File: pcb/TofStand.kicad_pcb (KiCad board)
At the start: 2 copper layers, 38.2 x 72.9 mm, 77 parts, among them SW2 SWITCH_H, U1 L6470, U2 USBLC6

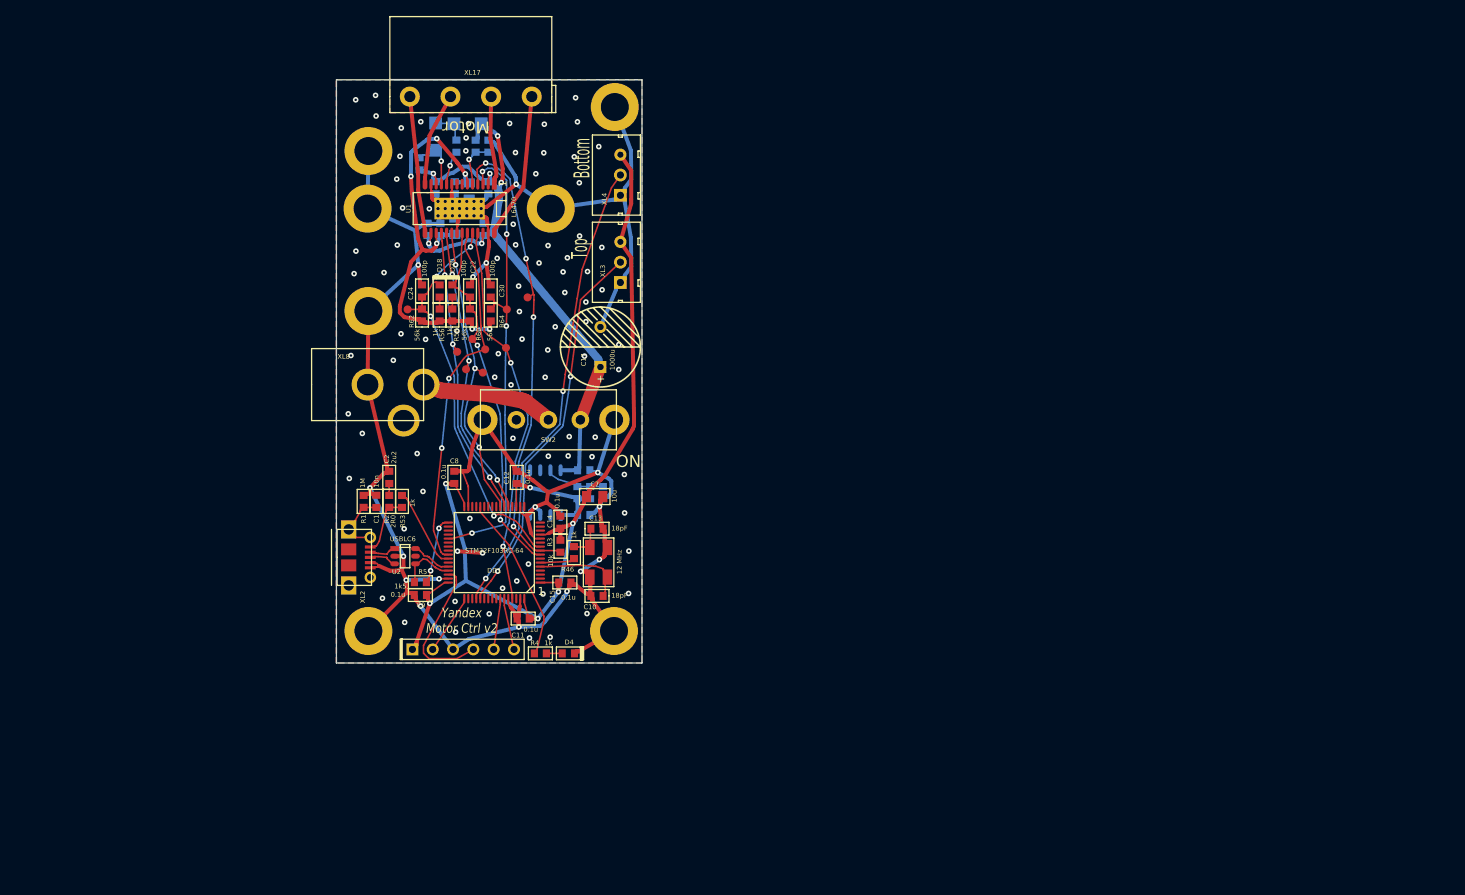
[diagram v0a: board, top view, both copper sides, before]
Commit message: PCB sent to factory
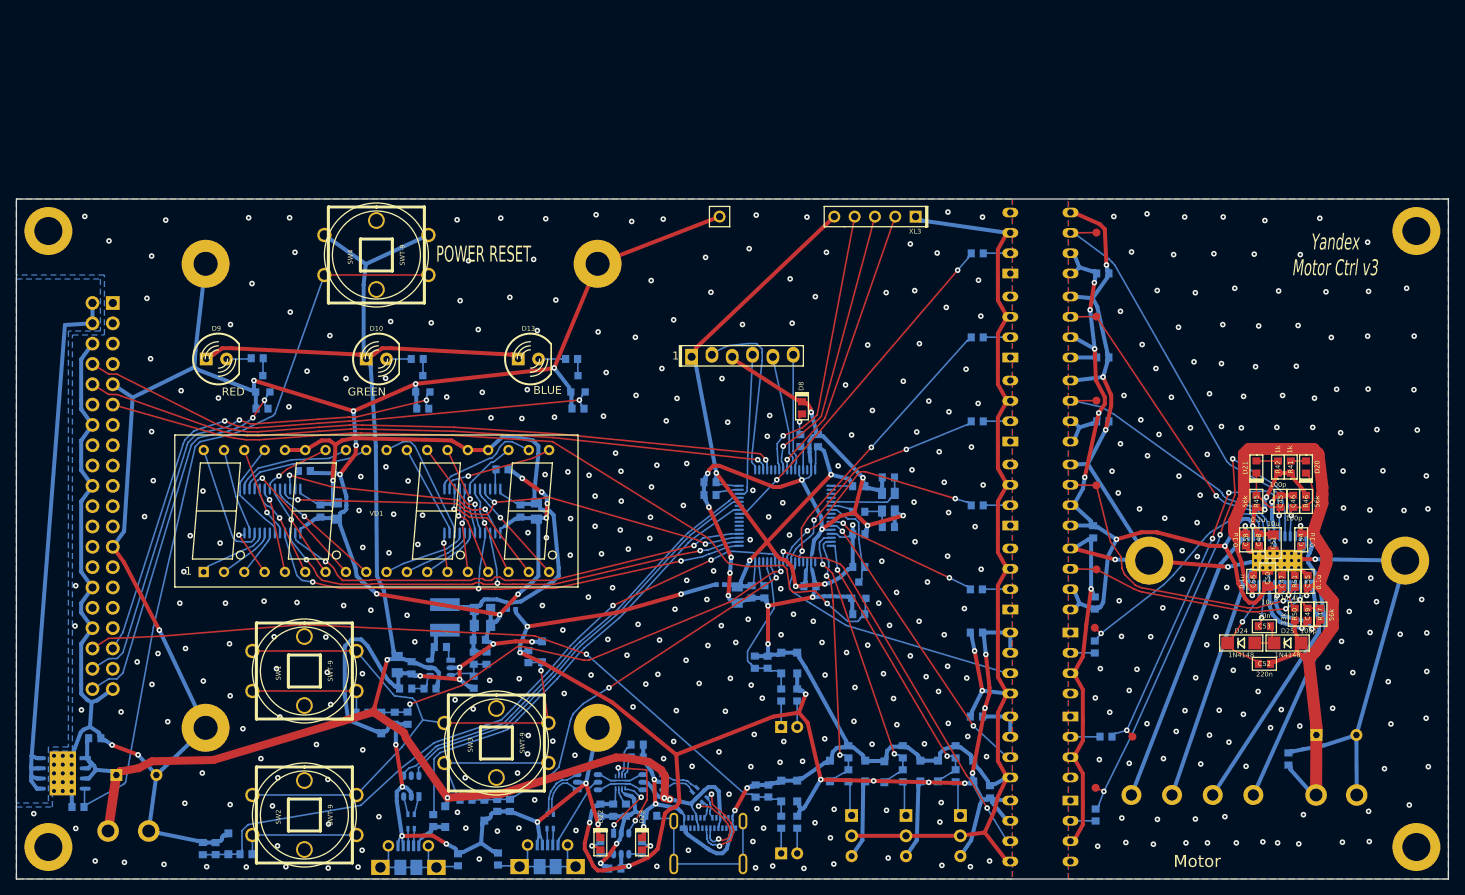
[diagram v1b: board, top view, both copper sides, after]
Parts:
- removed HOLE10, HOLE8: HOLE_METALLED, PCB:Hole3_5_out6mm
- removed R52: 12k, Resistors:RES_0603
- removed R53, R56, R58: 1k, Resistors:RES_0603
- removed R60, R62, R64: 56k, Resistors:RES_0603
- removed R68: 33k, Resistors:RES_0603
- removed R69: 4k7, Resistors:RES_0603
- removed TP4: TESTPOINT, PCB:TESTPOINT_1MM
- removed XL17: CONN_4, Connectors:TermiBlockHeader_508_x4_R
- added C20: 10u, Capacitors:CAP_0805, B.Cu at (86.3, 111.3)
- added C21: 10u, Capacitors:CAP_0805, B.Cu at (86.3, 109.3)
- added C23: 0.1u, Capacitors:CAP_0603_Silks, B.Cu at (120.4, 132.0)
- added C25: 0.1u, Capacitors:CAP_0603_Silks, B.Cu at (76.9, 122.9)
- added C28: 0.1u, Capacitors:CAP_0603_Silks, B.Cu at (163.8, 67.3)
- added C29: 0.1u, Capacitors:CAP_0603_Silks, B.Cu at (163.8, 77.8)
- added C3: 0.1u, Capacitors:CAP_0603_Silks, B.Cu at (37.8, 125.4)
- added C31: 0.1u, Capacitors:CAP_0603_Silks, B.Cu at (149.7, 132.1)
- added C34: 0.1u, Capacitors:CAP_0603_Silks, B.Cu at (162.6, 99.6)
- added C35: 0.1u, Capacitors:CAP_0603_Silks, B.Cu at (162.8, 108.5)
- added C38: 0.1u, Capacitors:CAP_0603_Silks, B.Cu at (105.6, 126.2)
- added C39: 10u, Capacitors:CAP_0805, B.Cu at (68.0, 97.0)
- added C4: 18pF, Capacitors:CAP_0603_Silks, B.Cu at (137.0, 99.0)
- added C41: 1u, Capacitors:CAP_0603_Silks, B.Cu at (102.8, 141.7)
- added C43: 0.1u, Capacitors:CAP_0603_Silks, B.Cu at (104.2, 134.4)
- added C45: 100p, Capacitors:CAP_0603_Silks, F.Cu at (186.0, 95.8)
- added C47: 0.1u, Capacitors:CAP_0603_Silks, F.Cu at (186.2, 105.8)
- added C48: 0.1u, Capacitors:CAP_0603_Silks, F.Cu at (183.3, 100.6)
- added C49: 100p, Capacitors:CAP_0603_Silks, F.Cu at (189.4, 109.9)
- added C5: 0.1u, Capacitors:CAP_0603_Silks, B.Cu at (119.9, 107.1)
- added C50: 10u, Capacitors:CAP_0805, F.Cu at (184.4, 105.4)
- added C51: 10u, Capacitors:CAP_0805, F.Cu at (185.1, 101.0)
- added C52: 220n, Capacitors:CAP_0603_Silks, F.Cu at (184.0, 116.1)
- added C53: 10n, Capacitors:CAP_0603_Silks, F.Cu at (184.0, 111.4)
- added C54: 0.1u, Capacitors:CAP_0603_Silks, F.Cu at (188.6, 100.6)
- added C55: 0.1u, Capacitors:CAP_0603_Silks, F.Cu at (189.4, 105.8)
- added C56: 0.1u, Capacitors:CAP_0603_Silks, F.Cu at (182.6, 105.8)
- added C57: 1000u, Capacitors:CAP_10xxR, B.Cu at (193.0, 125.0)
- added C58: 0.1u, Capacitors:CAP_0603_Silks, F.Cu at (181.7, 100.6)
- added C59: 0.1u, Capacitors:CAP_0603_Silks, B.Cu at (187.0, 128.0)
- added C6: 1000u, Capacitors:CAP_10xxR, B.Cu at (43.0, 130.0)
- added D1: PESD3V3, Diodes:SOD323, B.Cu at (134.1, 129.5)
- added D10: LED, LEDs:LED_Through-Hole-5mm, F.Cu at (73.0, 78.0)
- added D11: PESD3V3, Diodes:SOD323, B.Cu at (123.6, 132.0)
- added D12: PESD3V3, Diodes:SOD323, B.Cu at (125.6, 132.0)
- added D13: LED, LEDs:LED_Through-Hole-5mm, F.Cu at (92.0, 78.0)
- added D14: PESD3V3, Diodes:SOD323, B.Cu at (93.7, 114.6)
- added D15: PESD3V3, Diodes:SOD323, B.Cu at (73.6, 123.5)
- added D16: PESD3V3, Diodes:SOD323, B.Cu at (54.5, 138.6)
- added D17: PESD3V3, Diodes:SOD323, B.Cu at (86.5, 134.4)
- added D19: PESD3V3, Diodes:SOD323, B.Cu at (125.6, 116.0)
- added D2: PESD3V3, Diodes:SOD323, B.Cu at (141.0, 129.5)
- added D21: LED, LEDs:LED_0603, F.Cu at (183.0, 91.5)
- added D22: LED, LEDs:LED_0603, F.Cu at (101.0, 138.6)
- added D24: 1N4148, Diodes:SOD80C, F.Cu at (181.1, 113.5)
- added D3: PESD3V3, Diodes:SOD323, B.Cu at (147.6, 129.5)
- added D5: PESD3V3, Diodes:SOD323, B.Cu at (129.7, 129.5)
- added D6: PESD3V3, Diodes:SOD323, B.Cu at (136.5, 129.6)
- added D7: PESD3V3, Diodes:SOD323, B.Cu at (143.2, 129.5)
- added D8: LED, LEDs:LED_0603, F.Cu at (126.2, 84.1)
- added D9: LED, LEDs:LED_Through-Hole-5mm, F.Cu at (53.0, 78.0)
- added DA2: Optocoupler_6N137, DIP:DIP-8_296_ELL, B.Cu at (156.0, 116.0)
- added DA3: Optocoupler_6N137, DIP:DIP-8_296_ELL, B.Cu at (156.0, 63.5)
- added DA4: Optocoupler_6N137, DIP:DIP-8_296_ELL, B.Cu at (156.0, 74.0)
- added DA5: Optocoupler_6N137, DIP:DIP-8_296_ELL, B.Cu at (156.0, 84.5)
- added DA6: Optocoupler_6N137, DIP:DIP-8_296_ELL, B.Cu at (156.0, 137.0)
- added DA7: Optocoupler_6N137, DIP:DIP-8_296_ELL, B.Cu at (156.0, 126.5)
- added DA8: Optocoupler_6N137, DIP:DIP-8_296_ELL, B.Cu at (156.0, 95.0)
- added DA9: Optocoupler_6N137, DIP:DIP-8_296_ELL, B.Cu at (156.0, 105.5)
- added DD2: ICN2595, SO_DIL_TSSOP:TSSOP24_150_0635, B.Cu at (60.0, 97.0)
- added DD3: ICN2595, SO_DIL_TSSOP:TSSOP24_150_0635, B.Cu at (85.0, 97.0)
- added DD4: 74LVC2G17, SOT:SOT23-6, B.Cu at (103.6, 138.6)
- added DD5: TUSB211, QFN_DFN:X2QFN_12, B.Cu at (103.5, 130.9)
- added HOLE3: HOLE_METALLED, PCB:Hole3_5_out6mm, F.Cu at (203.0, 62.0)
- added L1: BLM21PG221SN1D, Inductors:IND_0603, B.Cu at (83.2, 140.6)
- added L2: BLM15AG102, Inductors:IND_0402, B.Cu at (116.0, 106.2)
- added L3: 90R, Inductors:DLW21SN, B.Cu at (77.3, 135.8)
- added L4: 2R2, Inductors:IND_1515, B.Cu at (81.6, 110.3)
- added L5: Choke, Inductors:IND_0402, B.Cu at (89.9, 109.3)
- added L6: BLM21PG221SN1D, Inductors:IND_0603, B.Cu at (107.3, 135.1)
- added L7: 90R, Inductors:DLW21SN, B.Cu at (113.4, 132.5)
- added L8: 90R, Inductors:DLW21SN, B.Cu at (94.7, 135.8)
- added L9: BLM21PG221SN1D, Inductors:IND_0603, B.Cu at (88.2, 140.5)
- added Q1: 2N7002, SOT:SOT23-3, B.Cu at (58.8, 81.1)
- added Q2: 2N7002, SOT:SOT23-3, B.Cu at (78.8, 81.1)
- added Q3: 2N7002, SOT:SOT23-3, B.Cu at (98.2, 81.1)
- added Q4: IRF9321, SO_DIL_TSSOP:SO8HEATSINK, B.Cu at (33.8, 129.8)
- added Q5: 2N7002, SOT:SOT23-3, B.Cu at (133.3, 106.9)
- added R10: 22k, Resistors:RES_0603, B.Cu at (85.2, 118.4)
- added R11: 100k, Resistors:RES_0603, B.Cu at (78.8, 84.2)
- added R12: 1k, Resistors:RES_0603, B.Cu at (125.6, 135.9)
- added R13: 1k, Resistors:RES_0603, B.Cu at (123.6, 135.9)
- added R14: 1k, Resistors:RES_0603, B.Cu at (78.1, 78.0)
- added R15: 1k, Resistors:RES_0603, B.Cu at (80.1, 135.7)
- added R16: 100k, Resistors:RES_0603, B.Cu at (98.2, 84.2)
- added R17: 100k, Resistors:RES_0603, B.Cu at (122.0, 132.0)
- added R18: 1k, Resistors:RES_0603, B.Cu at (97.4, 78.0)
- added R19: 1k, Resistors:RES_0603, B.Cu at (92.0, 115.2)
- added R20: 1k, Resistors:RES_0603, B.Cu at (148.1, 64.8)
- added R21: 1k, Resistors:RES_0603, B.Cu at (148.1, 75.3)
- added R22: 1k, Resistors:RES_0603, B.Cu at (148.1, 85.8)
- added R23: 1k, Resistors:RES_0603, B.Cu at (71.2, 122.2)
- added R24: 1k, Resistors:RES_0603, B.Cu at (56.7, 139.9)
- added R25: 1k, Resistors:RES_0603, B.Cu at (84.2, 133.1)
- added R26: 10k, Resistors:RES_0603, B.Cu at (35.7, 134.0)
- added R27: 100k, Resistors:RES_0603, B.Cu at (75.3, 122.9)
- added R28: 100k, Resistors:RES_0603, B.Cu at (52.9, 139.2)
- added R29: 100k, Resistors:RES_0603, B.Cu at (88.1, 133.8)
- added R30: 1k, Resistors:RES_0603, B.Cu at (162.8, 114.0)
- added R31: 1k, Resistors:RES_0603, B.Cu at (125.6, 120.0)
- added R32: 1k, Resistors:RES_0603, B.Cu at (123.6, 120.0)
- added R33: 1k, Resistors:RES_0603, B.Cu at (148.1, 96.3)
- added R34: 1k, Resistors:RES_0603, B.Cu at (148.0, 106.8)
- added R35: 100k, Resistors:RES_0603, B.Cu at (121.9, 115.9)
- added R36: 1k, Resistors:RES_0603, B.Cu at (162.9, 135.0)
- added R37: 1k, Resistors:RES_0603, B.Cu at (164.2, 125.2)
- added R38: 1k, Resistors:RES_0603, B.Cu at (64.0, 92.0)
- added R39: 1k, Resistors:RES_0603, B.Cu at (88.7, 91.8)
- added R40: 3k9, Resistors:RES_0603, B.Cu at (105.6, 127.8)
- added R41: 1k, Resistors:RES_0603, F.Cu at (187.3, 91.5)
- added R42: 1k, Resistors:RES_0603, F.Cu at (185.7, 91.5)
- added R43: 1k, Resistors:RES_0603, B.Cu at (101.0, 139.1)
- added R44: 1k, Resistors:RES_0603, B.Cu at (106.2, 139.1)
- added R45: 56k, Resistors:RES_0603, F.Cu at (183.0, 95.8)
- added R47: 56k, Resistors:RES_0603, F.Cu at (191.0, 109.9)
- added R48: 100k, Resistors:RES_0603, B.Cu at (133.3, 109.9)
- added R49: 10k, Resistors:RES_0603, B.Cu at (133.3, 104.0)
- added R50: 33k, Resistors:RES_0603, F.Cu at (187.8, 109.9)
- added R6: 1k, Resistors:RES_0603, B.Cu at (126.0, 88.2)
- added R7: 100k, Resistors:RES_0603, B.Cu at (58.7, 84.2)
- added R8: 1k, Resistors:RES_0603, B.Cu at (58.1, 77.9)
- added R9: 100k, Resistors:RES_0603, B.Cu at (85.2, 115.4)
- added SW1: SWT-9, BtnsSwitches:BTN_SWT9, F.Cu at (64.0, 117.0)
- added SW3: SWT-9, BtnsSwitches:BTN_SWT9, F.Cu at (88.0, 126.0)
- added SW4: SWT-9, BtnsSwitches:BTN_SWT9, F.Cu at (73.0, 65.0)
- added U3: USBLC6, SOT:SOT23-6, B.Cu at (99.4, 130.9)
- added U4: L6470, SO_DIL_TSSOP:HTSSOP28, B.Cu at (185.6, 103.2)
- added VCap1: 2.2u, Capacitors:CAP_0603_Silks, B.Cu at (121.5, 107.1)
- added VCap2: 2.2u, Capacitors:CAP_0603_Silks, B.Cu at (114.7, 95.0)
- added VD1: 7SEGx4_CA, Display:7Segx4, F.Cu at (73.0, 97.0)
- added XL10: CONN_2, Connectors:WB-02(MW-2M), B.Cu at (124.6, 124.0)
- added XL11: RASPBERRY_3B, Installation:RaspberryPi3, B.Cu at (40.0, 71.0)
- added XL12: CONN_4, Connectors:TermiBlockHeader_508_x4_R, B.Cu at (175.0, 132.5)
- added XL13: USB_MICRO, Connectors:USBmicro_MOLEX_1050170001, B.Cu at (94.4, 142.9)
- added XL14: CONN_2, Connectors:2ZHDRC-02P, B.Cu at (193.0, 132.5)
- added XL15: CONN_1, Connectors:PLS-1Rnd, B.Cu at (115.9, 60.2)
- added XL5: CONN_3, Connectors:W03_Pitch_2d54, B.Cu at (139.2, 137.6)
- added XL6: CONN_3, Connectors:W03_Pitch_2d54, B.Cu at (146.0, 137.6)
- added XL7: USB_MICRO, Connectors:USBmicro_MOLEX_1050170001, B.Cu at (77.0, 143.0)
- added XL9: USB_C, Connectors:USB_C_MOLEX_1054500101, B.Cu at (114.5, 142.9)
- C1: value 10n -> 18pF; footprint Capacitors:CAP_0603 -> Capacitors:CAP_0603_Silks; moved to B.Cu
- C10: value 18pF -> 10nF; footprint Capacitors:CAP_0603 -> Capacitors:CAP_0603_Silks; moved to B.Cu
- C11, C9: value 0.1u -> 10nF; footprint Capacitors:CAP_0603 -> Capacitors:CAP_0603_Silks; moved to B.Cu
- C12, C8: footprint Capacitors:CAP_0603 -> Capacitors:CAP_0603_Silks; moved to B.Cu
- C13: value 18pF -> 10u; footprint Capacitors:CAP_0603 -> Capacitors:CAP_0805; moved to B.Cu
- C14, C15: value 0.1u -> 1u; footprint Capacitors:CAP_0603 -> Capacitors:CAP_0603_Silks; moved to B.Cu
- C16, C26, C27: footprint Capacitors:CAP_0603 -> Capacitors:CAP_0603_Silks
- C17: value 1000u -> 0.1u; footprint Capacitors:CAP_10xxR -> Capacitors:CAP_0603_Silks; moved to B.Cu
- C18: value 1000pF -> 0.1u; footprint Capacitors:CAP_0603 -> Capacitors:CAP_0603_Silks
- C19: value 1u -> 27pF; footprint Capacitors:CAP_0603 -> Capacitors:CAP_0603_Silks
- C2: value 2u2 -> 10u; footprint Capacitors:CAP_0603 -> Capacitors:CAP_0805; moved to B.Cu
- C22, C24, C30: value 100p -> 0.1u; footprint Capacitors:CAP_0603 -> Capacitors:CAP_0603_Silks; moved to B.Cu
- C32, C33: value 10u -> 0.1u; footprint Capacitors:CAP_0805 -> Capacitors:CAP_0603_Silks
- C36: value 220n -> 0.1u; footprint Capacitors:CAP_0603 -> Capacitors:CAP_0603_Silks
- C37: value 10n -> 0.1u; footprint Capacitors:CAP_0603 -> Capacitors:CAP_0603_Silks
- C40: value 0.1u -> 10u; footprint Capacitors:CAP_0603 -> Capacitors:CAP_0805
- C42: value 0.1u -> 10n; footprint Capacitors:CAP_0603 -> Capacitors:CAP_0603_Silks
- C44: value 0.1u -> 1u; footprint Capacitors:CAP_0603 -> Capacitors:CAP_0603_Silks
- C46: value 0.1u -> 100p; footprint Capacitors:CAP_0603 -> Capacitors:CAP_0603_Silks; moved to F.Cu
- C7: value 10u -> 0.1u; footprint Capacitors:CAP_0805 -> Capacitors:CAP_0603_Silks; moved to B.Cu
- D18: value LED -> PESD3V3; footprint LEDs:LED_0603 -> Diodes:SOD323; moved to B.Cu
- D23: value 1N4148 -> LED; footprint Diodes:SOD80C -> LEDs:LED_0603; moved to F.Cu
- D25: moved to F.Cu
- D4: value LED -> PMEG2020; footprint LEDs:LED_0603 -> Diodes:SOD323; moved to B.Cu
- DA1: value LP2951 -> SY8120; footprint SO_DIL_TSSOP:SO8_150MIL -> SOT:SOT23-6
- DD1: value STM32F103RC-64 -> STM32F205Rx-64; moved to B.Cu
- R1: value 1M -> 1k; moved to B.Cu
- R2: value 2R0 -> 1k; moved to B.Cu
- R3: value 10k -> 1k; moved to B.Cu
- R4, U2, XL4: moved to B.Cu
- R46: value 1k -> 56k
- R5: value 1k5 -> 56k; moved to B.Cu
- R51: value 20k -> 4k7; moved to F.Cu
- SW2: value SWITCH_H -> SWT-9; footprint BtnsSwitches:SW_SS9 -> BtnsSwitches:BTN_SWT9
- U1: value L6470 -> USBLC6; footprint SO_DIL_TSSOP:HTSSOP28 -> SOT:SOT23-6; moved to B.Cu
- XL1: value CONN_6 -> CONN_2; footprint Connectors:PLS-6 -> Connectors:2ZHDRC-02P; moved to B.Cu
- XL2: value USB_MICRO -> CONN_6; footprint Connectors:USBmicro_MOLEX_1050170001 -> Connectors:PLS-6_LOCK
- XL3: value CONN_3 -> CONN_5; footprint Connectors:W03_Pitch_2d54 -> Connectors:PLS-5
- XL8: value BARREL_SOCKET -> CONN_2; footprint Connectors:Barrel -> Connectors:WB-02(MW-2M); moved to B.Cu
- XTAL1: footprint Quartz:0503x4-4 -> Quartz:03225C4; moved to B.Cu
- moved HOLE6 134.4 mm to (203.0, 139.0), turned to 0 degrees
- moved HOLE2 129.9 mm to (201.6, 103.2)
- moved D25 121.3 mm to (186.9, 113.5)
- moved C46 113.4 mm to (187.6, 95.8)
- moved D20 108.9 mm to (189.2, 91.5), turned to -90 degrees
- moved TP3 104.7 mm to (162.9, 131.6), turned to 0 degrees
- moved HOLE1 102.5 mm to (169.6, 103.2)
- moved TP1 96.3 mm to (167.5, 125.2), turned to 0 degrees
- moved HOLE4 95.8 mm to (32.0, 139.0)
- moved D23 92.1 mm to (106.2, 138.6)
- moved R46 91.7 mm to (189.2, 95.8), turned to -90 degrees
- moved C32 91.3 mm to (148.0, 122.7), turned to 180 degrees
- moved R51 90.4 mm to (187.8, 105.8)
- moved C26 88.4 mm to (51.3, 139.2), turned to 90 degrees
- moved XL4 87.5 mm to (132.4, 137.6), turned to -90 degrees
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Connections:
- C1 pad 1: GND -> Net-(C1-Pad1)
- C1 pad 2: Net-(C1-Pad2) -> GND
- C10 pad 1: Net-(C10-Pad1) -> /ENDSTOP_BOT
- C11 pad 1: +3v3 -> /ENDSTOP_TOUCH
- C12 pad 1: +3v3 -> PwrMCU
- C13 pad 1: Net-(C13-Pad1) -> +5v
- C14 pad 1: +3v3 -> +5v
- C15 pad 1: +3v3 -> PwrMCU
- C16 pad 1: +12v -> PwrMCU
- C17 pad 1: +12v -> Net-(C13-Pad1)
- C18 pad 1: +3v3 -> Net-(C19-Pad1)
- C18 pad 2: Net-(C18-Pad2) -> Net-(C19-Pad2)
- C19 pad 1: +3v3 -> /PWR_LEDS
- C19 pad 2: GND -> Net-(C23-Pad2)
- C2 pad 1: Net-(C2-Pad1) -> PwrMCU
- C22 pad 1: /BUSY/SYNC_1 -> /PWR_LEDS
- C24 pad 1: /FLAG_1 -> +3v3
- C26 pad 1: /Vdd1 -> /BtnDown
- C27 pad 1: /Vdd1 -> /BtnFast
- C30 pad 1: /STBY/RST -> VCC
- C30 pad 2: GND -> GNDPWR
- C32 pad 1: /Vdd1 -> +3v3
- C33 pad 1: /Vdd1 -> /ChClosed
- C36 pad 1: Net-(C36-Pad1) -> GND
- C36 pad 2: +12v -> /PWR_LEDS
- C37 pad 1: Net-(C37-Pad1) -> GND
- C37 pad 2: Net-(C37-Pad2) -> /PWR_LEDS
- C40 pad 1: +12v -> GND
- C40 pad 2: GND -> /PWR_LEDS
- C42 pad 1: +12v -> GND
- C42 pad 2: GND -> +3v3
- C44 pad 1: +12v -> GND
- C44 pad 2: GND -> +3v3
- C46 pad 1: +12v -> /FLAG
- C46 pad 2: GND -> GNDPWR
- C7 pad 1: +3v3 -> PwrMCU
- C8 pad 1: +3v3 -> PwrMCU
- C9 pad 1: +3v3 -> /ENDSTOP_TOP
- D18 pad A: Net-(D18-PadA) (its old number) -> GND
- D18 pad C: /FLAG_1 -> /ChClosed
- D20 pad C: /BUSY/SYNC_1 -> /FLAG
- D23 pad A: Net-(C37-Pad1) -> Net-(D21-PadA)
- D23 pad C: Net-(C36-Pad1) -> GND
- D4 pad A: Net-(D4-PadA) -> /5V_USB
- D4 pad C: GND -> +5v
- DA1 pad 1: +3v3 -> Net-(C19-Pad1)
- DA1 pad 2: (no net) -> GND
- DA1 pad 3: GND -> Net-(C23-Pad2)
- DA1 pad 4: GND -> Net-(C13-Pad1)
- DA1 pad 5: (no net) -> +5v
- DA1 pad 6: (no net) -> Net-(C19-Pad2)
- DD1 pad 1: +3v3 -> PwrMCU
- DD1 pad 10: /FLAG_1 -> /STBY/RST_MCU
- DD1 pad 11: (no net) -> /BUSY/SYNC_MCU
- DD1 pad 13: +3v3 -> PwrMCU
- DD1 pad 14: (no net) -> /ENDSTOP_BOT
- DD1 pad 15: (no net) -> /ENDSTOP_TOP
- DD1 pad 16: (no net) -> /ENDSTOP_TOUCH
- DD1 pad 19: +3v3 -> PwrMCU
- DD1 pad 21: /MOTOR_SCK -> /MOTOR_SCK_MCU
- DD1 pad 22: /MOTOR_MISO -> /MOTOR_MISO_MCU
- DD1 pad 23: /MOTOR_MOSI -> /MOTOR_MOSI_MCU
- DD1 pad 24: (no net) -> /SW_MCU
- DD1 pad 25: (no net) -> /FLAG_MCU
- DD1 pad 26: (no net) -> /BtnUp
- DD1 pad 27: (no net) -> /BtnDown
- DD1 pad 28: Net-(DD1-Pad28) -> /BtnFast
- DD1 pad 29: (no net) -> /ChClosed
- DD1 pad 31: GND -> Net-(DD1-Pad31)
- DD1 pad 32: +3v3 -> PwrMCU
- DD1 pad 33: /USB_PULLUP -> /LATCH
- DD1 pad 34: (no net) -> /CLK
- DD1 pad 35: (no net) -> /OUT_EN
- DD1 pad 36: (no net) -> /DATA_IN1
- DD1 pad 37: /STBY/RST -> (no net)
- DD1 pad 41: /MOTOR_CS -> /MOTOR_CS_MCU
- DD1 pad 47: GND -> Net-(DD1-Pad47)
- DD1 pad 48: +3v3 -> PwrMCU
- DD1 pad 5: Net-(C10-Pad1) -> Net-(C1-Pad1)
- DD1 pad 51: (no net) -> /MCU_TX_RPI_RX
- DD1 pad 52: /ENDSTOP_BOT -> /MCU_RX_RPI_TX
- DD1 pad 53: /ENDSTOP_TOP -> (no net)
- DD1 pad 55: (no net) -> /PB5
- DD1 pad 56: (no net) -> /PB4
- DD1 pad 57: (no net) -> /PB3
- DD1 pad 61: /STEP_CLK_1 -> Net-(DD1-Pad61)
- DD1 pad 64: +3v3 -> PwrMCU
- DD1 pad 7: (no net) -> /MCU_RESET
- DD1 pad 8: /BUSY/SYNC_1 -> (no net)
- DD1 pad 9: /SW_1 -> (no net)
- HOLE1 pad H: GND -> GNDPWR
- HOLE2 pad H: GND -> GNDPWR
- HOLE4 pad H: GND -> (no net)
- HOLE5 pad H: GND -> (no net)
- HOLE6 pad H: GND -> (no net)
- R1 pad 1: Net-(C1-Pad2) -> /ENDSTOP_TOP
- R1 pad 2: GND -> Net-(R1-Pad2)
- R2 pad 1: /5V_USB -> /ENDSTOP_BOT
- R2 pad 2: Net-(C2-Pad1) -> Net-(R2-Pad2)
- R3 pad 1: +3v3 -> /ENDSTOP_TOUCH
- R3 pad 2: /SW_1 -> Net-(R3-Pad2)
- R4 pad 1: Net-(DD1-Pad28) -> Net-(DD1-Pad6)
- R4 pad 2: Net-(D4-PadA) -> Net-(C4-Pad1)
- R46 pad 1: Net-(DD1-Pad6) -> VCC
- R46 pad 2: Net-(C13-Pad1) -> /FLAG
- R5 pad 1: /USB_D+ -> Net-(C13-Pad1)
- R5 pad 2: /USB_PULLUP -> +5v
- R51 pad 1: +3v3 -> /ADC_1
- R51 pad 2: Net-(C18-Pad2) -> GNDPWR
- SW2 pad 1: +12v -> Net-(D14-PadC)
- SW2 pad 2: /PWR_IN -> Net-(R24-Pad1)
- SW2 pad H: GND -> (no net)
- TP1 pad 1: /BUSY/SYNC_1 -> /BUSY/SYNC
- TP2 pad 1: /SW_1 -> /SW
- TP3 pad 1: /FLAG_1 -> /FLAG
- TP5 pad 1: /STBY/RST -> /STBY/RST
- U1 pad 1: /OUT1_1A -> Net-(L1-Pad2)
- U1 pad 2: +12v -> GND
- U1 pad 3: /STBY/RST -> Net-(L1-Pad3)
- U1 pad 4: /SW_1 -> /USB_D+
- U1 pad 5: /ADC_1 -> (no net)
- U1 pad 6: /Vdd1 -> /USB_D-
- U2 pad 1: /DIN- -> Net-(L7-Pad2)
- U2 pad 3: /DIN+ -> Net-(L7-Pad3)
- U2 pad 4: /USB_D+ -> /USB2_D-
- U2 pad 5: (no net) -> +5v
- U2 pad 6: /USB_D- -> /USB2_D+
- XL1 pad 1: +3v3 -> GND
- XL1 pad 2: /SWCLK -> +5v
- XL2 pad 1: /5V_USB -> PwrMCU
- XL2 pad 2: /DIN- -> /SWCLK
- XL2 pad 3: /DIN+ -> GND
- XL2 pad 4: GND -> /SWDIO
- XL2 pad 5: GND -> /UART_TX
- XL3 pad 2: /ENDSTOP_TOP -> /PB3
- XL3 pad 3: +3v3 -> /PB4
- XL4 pad 1: GND -> Net-(R1-Pad2)
- XL4 pad 2: /ENDSTOP_BOT -> GND
- XTAL1 pad 1: Net-(C10-Pad1) -> Net-(C1-Pad1)
- XTAL1 pad 2: Net-(C13-Pad1) -> Net-(C4-Pad1)
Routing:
- net GND: track 316.4 -> 853.5 mm, vias 104 -> 346
- net +5v: track 0.00 -> 242.9 mm, vias 0 -> 4
- net GNDPWR: track 0.00 -> 220.6 mm, vias 0 -> 149
- net VCC: track 0.00 -> 140.3 mm, vias 0 -> 12
- net PwrMCU: track 0.00 -> 121.0 mm, vias 0 -> 6
- net /MCU_RESET_CTRL: track 0.00 -> 106.1 mm, vias 0 -> 1
- net /Btn: track 0.00 -> 95.7 mm, vias 0 -> 1
- net /PWR_LEDS: track 0.00 -> 93.9 mm, vias 0 -> 1
- net Net-(Q8-Pad4): track 0.00 -> 93.7 mm
- net /MCU_RX_RPI_TX: track 0.00 -> 87.9 mm, vias 0 -> 1
- net /BtnDown: track 0.00 -> 86.5 mm, vias 0 -> 2
- net /MCU_TX_RPI_RX: track 0.00 -> 86.1 mm, vias 0 -> 1
- net +3v3: track 136.9 -> 220.9 mm, vias 6 -> 13
- net /Green: track 0.00 -> 80.4 mm, vias 0 -> 2
- net Net-(D14-PadC): track 0.00 -> 76.3 mm, vias 0 -> 1
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- added copper zone on B.Cu, net /PWR_RPI
- added copper zone on B.Cu, net GNDPWR
- added copper zone on F.Cu, net GNDPWR
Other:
- board size 38.2 x 72.9 mm -> 179 x 85 mm
- rule via_min_size: 0.4 -> 0.7
- board text added: "BLUE"
- board text added: "GREEN"
- board text added: "POWER RESET"
- board text added: "RED"
- board text added: "Touch"
- board text added: "Yandex Motor Ctrl v3"
- board text removed: "ON"
- board text removed: "Yandex Motor Ctrl v2"
